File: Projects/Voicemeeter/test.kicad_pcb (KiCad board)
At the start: 2 copper layers, 348.5 x 271.7 mm, 225 parts, among them J501 Conn_01x08, J503 CONN_01X05, J504 CONN_01X02, J505 CONN_01X03, J506 CONN_01X02, J509 Screw_Terminal_1x02, SW201 SW_SPDT_6pin, SW202 SW_SPDT_6pin, SW203 SW_SPDT_6pin, SW204 SW_SPDT_6pin, SW205 SW_SPDT_6pin, SW206 SW_SPDT_6pin, SW207 SW_SPDT_6pin, SW208 SW_SPDT_6pin, SW209 SW_SPDT_6pin, SW210 SW_SPDT_6pin, SW211 SW_SPDT_6pin, SW212 SW_SPDT_6pin, SW213 SW_SPDT_6pin, SW214 SW_SPDT_6pin, SW215 SW_SPDT_6pin, SW216 SW_SPDT_6pin, SW217 SW_SPDT_6pin, SW218 SW_SPDT_6pin, SW219 SW_SPDT_6pin, SW220 SW_SPDT_6pin, SW221 SW_SPDT_6pin, SW222 SW_SPDT_6pin, SW223 SW_SPDT_6pin, SW224 SW_SPDT_6pin, SW225 SW_SPDT_6pin, SW226 SW_SPDT_6pin, SW227 SW_SPDT_6pin, SW228 SW_SPDT_6pin, SW229 SW_SPDT_6pin, SW230 SW_SPDT_6pin, SW231 SW_SPDT_6pin, SW232 SW_SPDT_6pin, SW233 SW_SPDT_6pin, SW234 SW_SPDT_6pin, SW235 SW_SPDT_6pin, SW236 SW_SPDT_6pin, SW237 SW_SPDT_6pin, SW238 SW_SPDT_6pin, SW239 SW_SPDT_6pin, SW240 SW_SPDT_6pin, SW241 SW_SPDT_6pin, SW242 SW_SPDT_6pin, SW243 SW_SPDT_6pin, SW244 SW_SPDT_6pin, SW245 SW_SPDT_6pin, SW246 SW_SPDT_6pin, SW247 SW_SPDT_6pin, SW248 SW_SPDT_6pin, SW249 SW_SPDT_6pin, SW250 SW_SPDT_6pin, SW251 SW_SPDT_6pin, SW252 SW_SPDT_6pin, SW253 SW_SPDT_6pin, SW254 SW_SPDT_6pin, SW255 SW_SPDT_6pin, SW501 SW_Push, U401 74HC4051, U402 74HC4051, U403 74HC4051, U404 74HC4051, U405 74HC4051, U406 74HC4051, U407 74HC4051, U408 74HC4051, U409 74HC4051, U410 74HC4051, U501 stm32f103-china-MS, U502 PC817

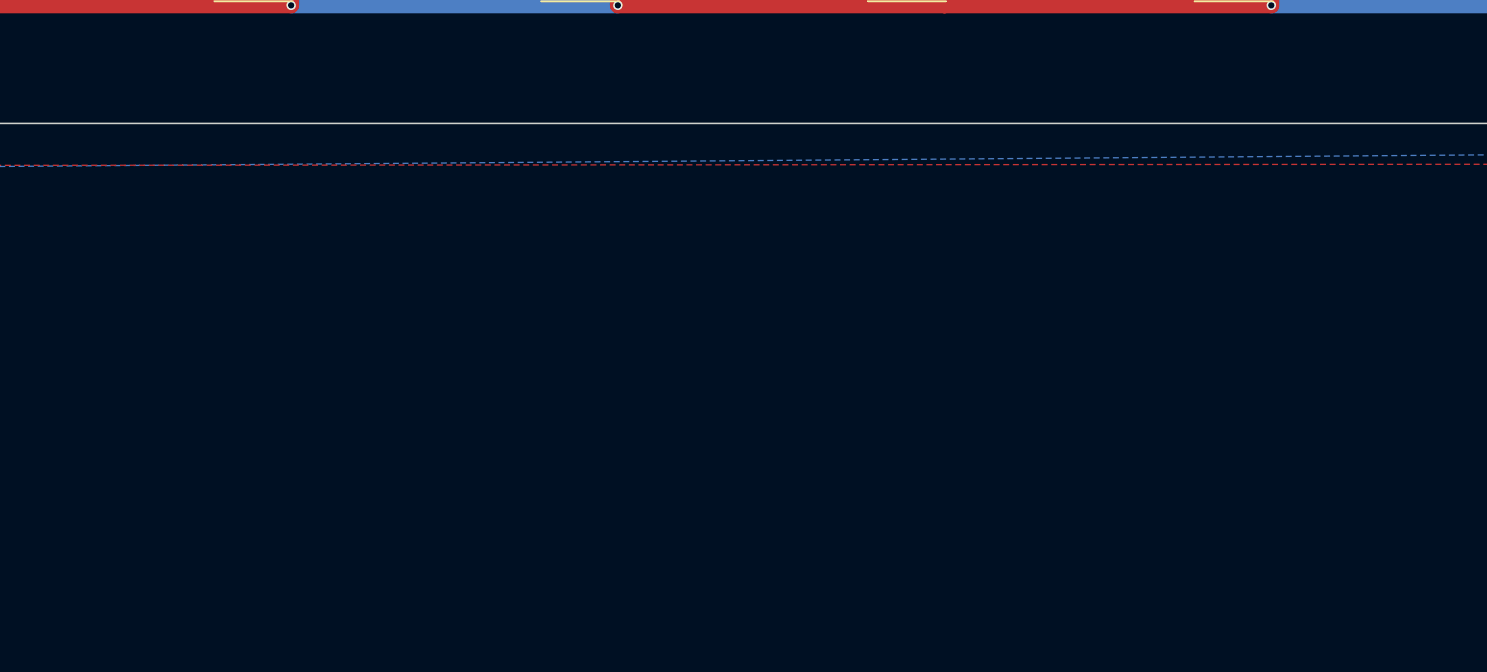
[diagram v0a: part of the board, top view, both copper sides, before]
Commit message: stuff
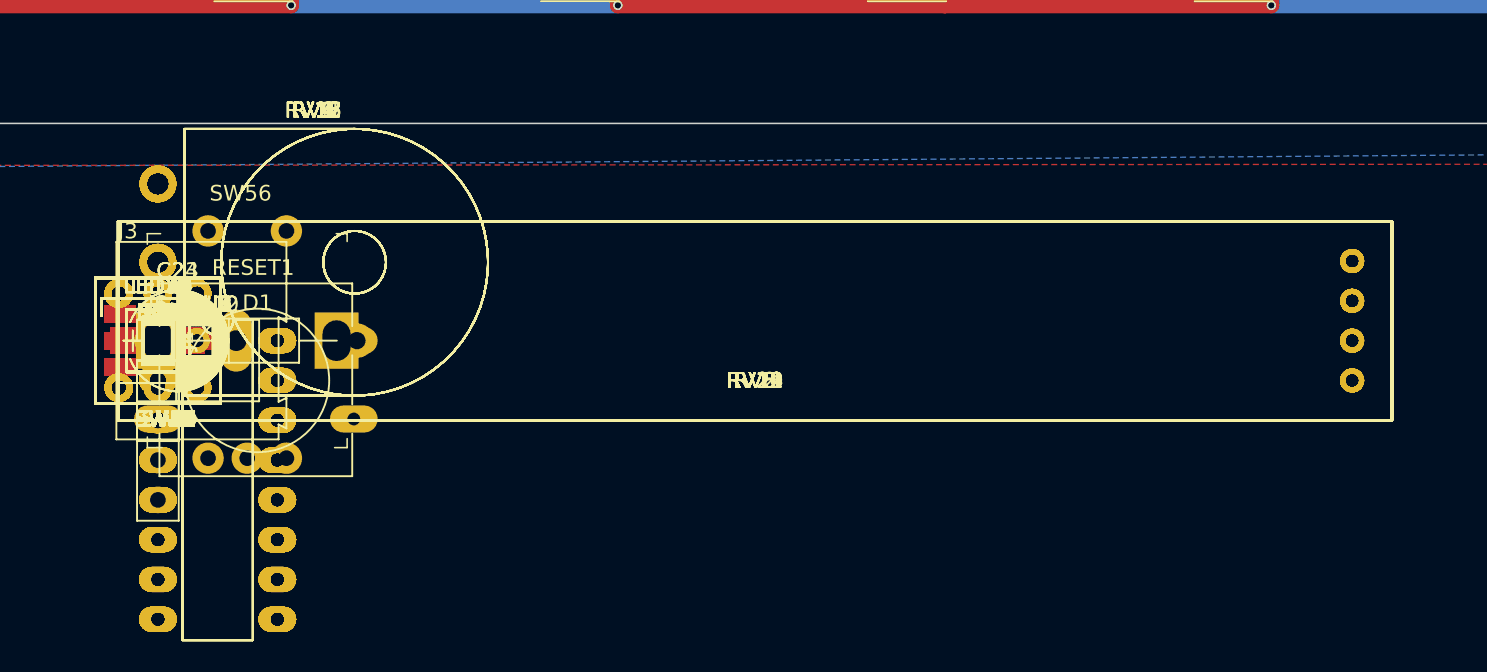
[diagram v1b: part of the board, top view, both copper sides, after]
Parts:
- added C1, C10, C11, C12, C13, C14, C15, C16, C17, C18, C19, C2, C20, C21, C22, C3, C4, C5, C6, C7, C8, C9: 10uF, Capacitors_SMD:C_1206_HandSoldering, F.Cu at (206.8, 256.4)
- added C23, C24: 220uF, Capacitors_THT:CP_Radial_D6.3mm_P2.50mm, F.Cu at (206.8, 256.4)
- added D1: D, Diodes_THT:D_DO-41_SOD81_P12.70mm_Horizontal, F.Cu at (206.8, 256.4)
- added J1: SPARE, Pin_Headers:Pin_Header_Straight_1x05_Pitch2.54mm, F.Cu at (206.8, 256.4)
- added J2, J4: GS2, MATHSTERK:SB2, F.Cu at (206.8, 256.4)
- added J3: Screw_Terminal_01x02, Connectors_Terminal_Blocks:TerminalBlock_Altech_AK300-2_P5.00mm, F.Cu at (206.8, 256.4)
- added J5: MIDI OUT, Pin_Headers:Pin_Header_Straight_1x03_Pitch2.54mm, F.Cu at (206.8, 256.4)
- added J6: MIDI IN, Pin_Headers:Pin_Header_Straight_1x02_Pitch2.54mm, F.Cu at (206.8, 256.4)
- added LED1, LED10, LED11, LED12, LED13, LED14, LED15, LED16, LED17, LED18, LED19, LED2, LED20, LED21, LED22, LED23, LED24, LED25, LED26, LED27, LED28, LED29, LED3, LED30, LED31, LED32, LED4, LED5, LED6, LED7, LED8, LED9: SK9822, LEDs:LED_RGB_5050-6, F.Cu at (206.8, 256.4)
- added R1, R10, R11, R12, R13, R14, R15, R16, R17, R18, R19, R2, R20, R21, R22, R23, R24, R25, R26, R27, R28, R29, R3, R30, R31, R32, R33, R34, R35, R36, R37, R38, R39, R4, R40, R41, R42, R43, R44, R45, R46, R47, R48, R49, R5, R50, R51, R52, R53, R54, R55, R6, R7, R8, R9: 10K, Resistors_SMD:R_1206_HandSoldering, F.Cu at (206.8, 256.4)
- added R56, R57, R58, R59, R60, R61, R62, R63, R64, R65, R66, R67, R68, R70, R71, R72, R73, R75, R77: 10k, Resistors_SMD:R_1206_HandSoldering, F.Cu at (206.8, 256.4)
- added R69, R76: 220R, Resistors_SMD:R_1206_HandSoldering, F.Cu at (206.8, 256.4)
- added R74: 330R, Resistors_SMD:R_1206_HandSoldering, F.Cu at (206.8, 256.4)
- added RESET1: SW_Push, Buttons_Switches_THT:SW_PUSH-12mm, F.Cu at (206.8, 256.4)
- added RV1, RV11, RV12, RV13, RV15, RV16, RV17, RV3, RV4, RV6, RV7, RV9: POT, Potentiometers:Potentiometer_Omeg_PC16PU_Horizontal, F.Cu at (206.8, 256.4)
- added RV10, RV14, RV18, RV19, RV2, RV20, RV21, RV22, RV5, RV8: SLIDEPOT, MATHSTERK:slidepot, F.Cu at (206.8, 256.4)
- added SW1, SW10, SW11, SW12, SW13, SW14, SW15, SW16, SW17, SW18, SW19, SW2, SW20, SW21, SW22, SW23, SW24, SW25, SW26, SW27, SW28, SW29, SW3, SW30, SW31, SW32, SW33, SW34, SW35, SW36, SW37, SW38, SW39, SW4, SW40, SW41, SW42, SW43, SW44, SW45, SW46, SW47, SW48, SW49, SW5, SW50, SW51, SW52, SW53, SW54, SW55, SW6, SW7, SW8, SW9: SW_SPDT_6pin, MATHSTERK:8mm_push_button, F.Cu at (206.8, 256.4)
- added SW56: PEC11R-4215F-S0024, MATHSTERK:Rotary_Encoder_Switched_PEC11R, F.Cu at (206.8, 256.4)
- added U1, U10, U2, U3, U4, U5, U6, U7, U8, U9: 74HC4051, Housings_DIP:DIP-16_W7.62mm_LongPads, F.Cu at (206.8, 256.4)
- added U12: PC817, Housings_DIP:DIP-4_W7.62mm, F.Cu at (206.8, 256.4)
